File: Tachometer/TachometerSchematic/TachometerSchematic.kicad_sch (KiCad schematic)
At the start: 4 parts, among them M1 Motor_DC, Q1 BC547

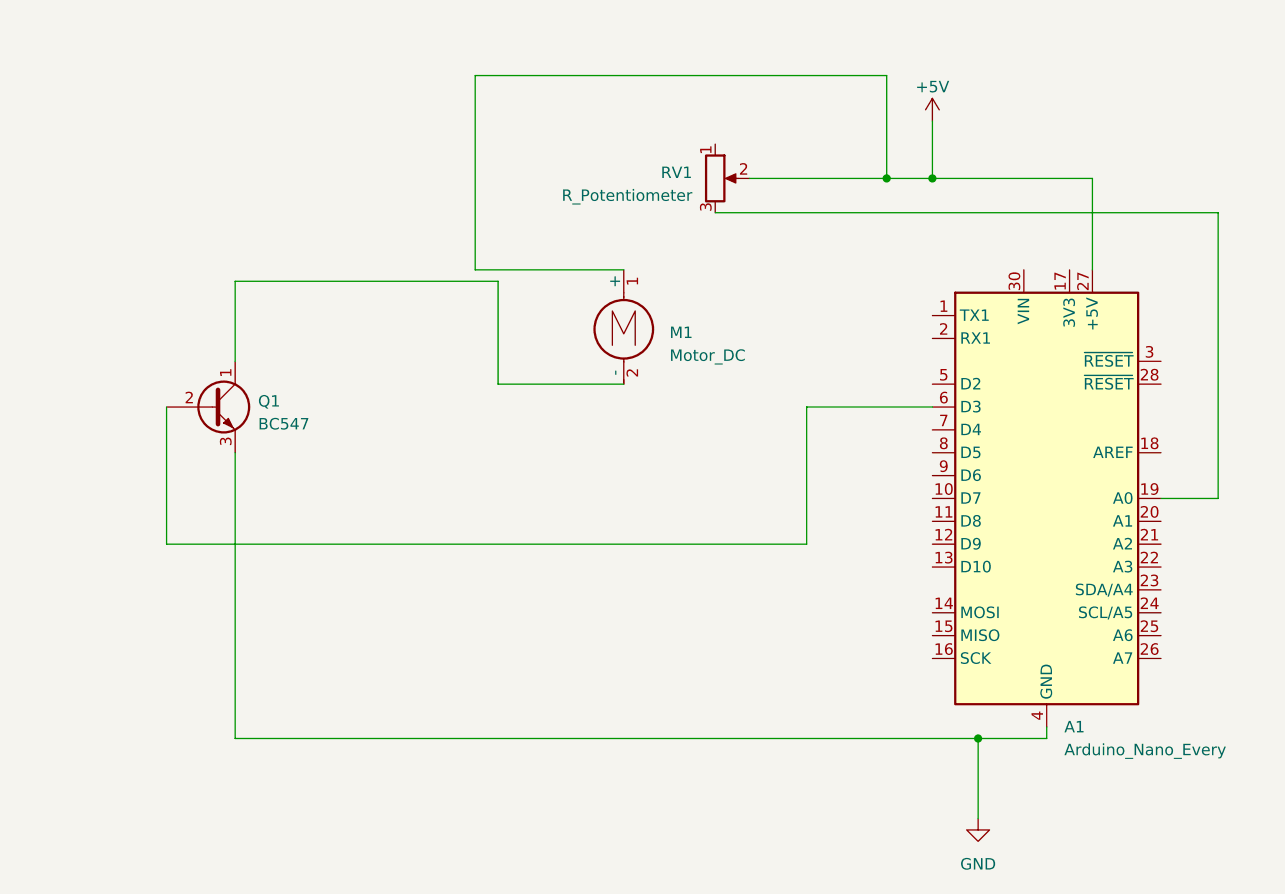
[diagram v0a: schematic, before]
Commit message: Signed-off-by: FCVEER <rik@veerhoek.nl>
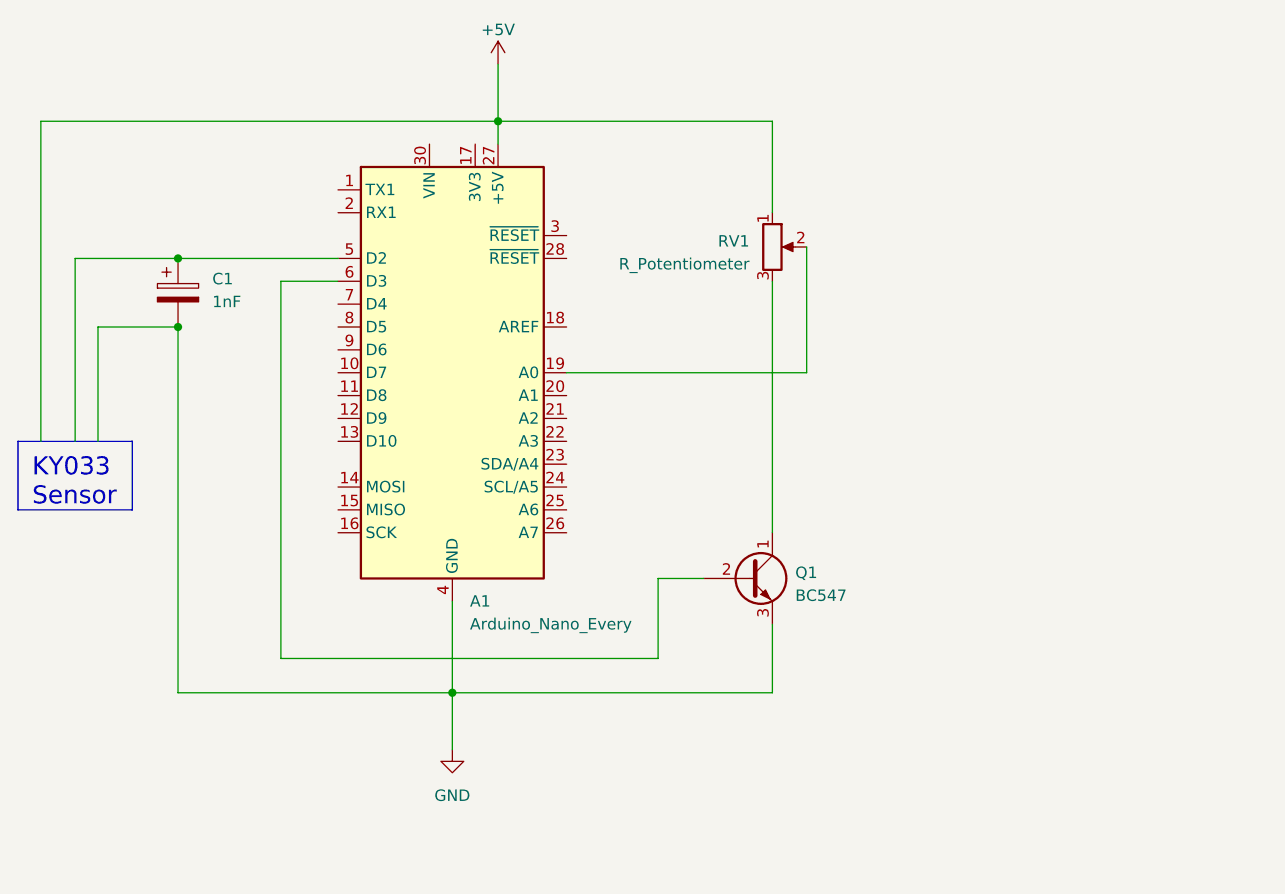
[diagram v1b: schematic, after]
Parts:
- removed M1: Motor_DC, symbol Motor:Motor_DC
- added C1: 1nF, symbol Device:C_Polarized
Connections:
- net +5V: now also RV1.1; no longer RV1.2
- net GND: now also C1.2
- net at A1.19 (A0): now also RV1.2; no longer RV1.3
- net at Q1.1 (C): now also RV1.3
- net at A1.5 (D2): now also C1.1

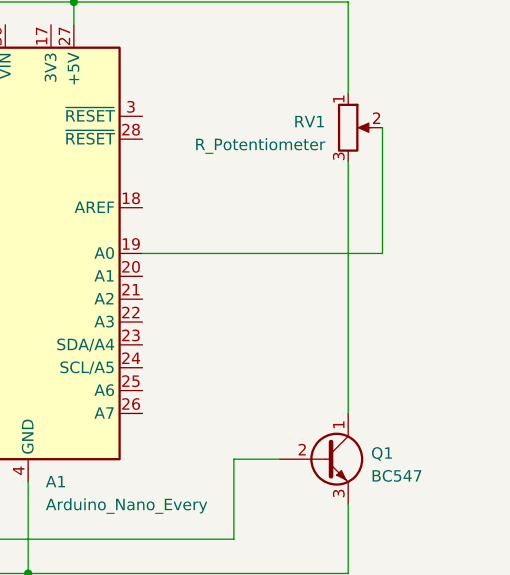
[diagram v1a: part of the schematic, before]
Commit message: Signed-off-by: FCVEER <rik@veerhoek.nl>
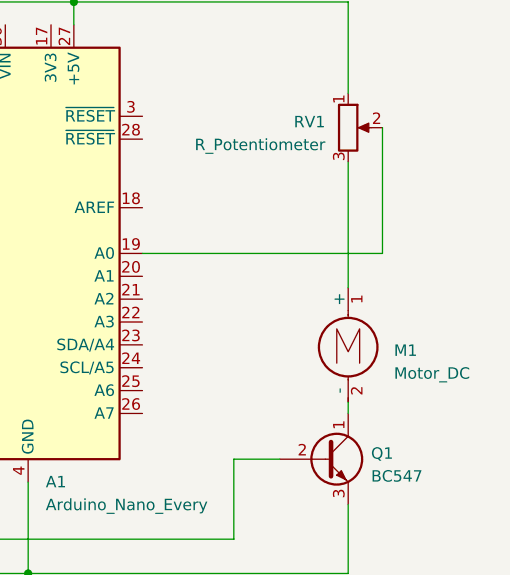
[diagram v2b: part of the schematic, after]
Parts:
- added M1: Motor_DC, symbol Motor:Motor_DC
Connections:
- net at RV1.3: now also M1.1 (+); no longer Q1.1 (C)
- new net: M1.2 (-), Q1.1 (C)
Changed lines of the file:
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@@
+    (stroke (width 0) (type default))
+  )
+  (wire (pts (xy 137.16 82.55) (xy 137.16 83.82))
     (stroke (width 0) (type default))
   )
@@
     (stroke (width 0) (type default))
   )
-  (wire (pts (xy 137.16 55.88) (xy 137.16 83.82))
+  (wire (pts (xy 137.16 55.88) (xy 137.16 69.85))
     (stroke (width 0) (type default))
   )
@@
     (effects (font (size 2 2) (color 0 0 0 1)) (justify left top))
   )
+  (symbol (lib_id "Motor:Motor_DC") (at 137.16 74.93 0) (unit 1)
+    (in_bom yes) (on_board yes) (dnp no) (fields_autoplaced)
+    (property "Reference" "M1" (at 142.24 76.835 0)
+      (effects (font (size 1.27 1.27)) (justify left))
+    )
+    (property "Value" "Motor_DC" (at 142.24 79.375 0)
+      (effects (font (size 1.27 1.27)) (justify left))
+    )
+    (property "Footprint" "" (at 137.16 77.216 0)
+      (effects (font (size 1.27 1.27)) hide)
+    )
+    (property "Datasheet" "~" (at 137.16 77.216 0)
+      (effects (font (size 1.27 1.27)) hide)
+    )
+    (pin "1")
+    (pin "2")
+    (instances
+      (project "TachometerSchematic"
+        (path "/96da9cfc-5e80-4b06-9459-77aeafd89275"
+          (reference "M1") (unit 1)
+        )
+      )
+    )
+  )
   (symbol (lib_id "Device:R_Potentiometer") (at 137.16 52.07 0) (unit 1)
